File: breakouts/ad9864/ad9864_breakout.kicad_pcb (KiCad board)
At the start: 4 copper layers, 44 x 39 mm, 82 parts, among them P101 CONN_01X02, P102 CONN_01X08, P103 CONN_02X08, U101 CONN_SMA, U102 CONN_SMA, U103 ad9864, U104 TXCO, U105 CONN_SMA, U106 CONN_SMA, U107 max2605

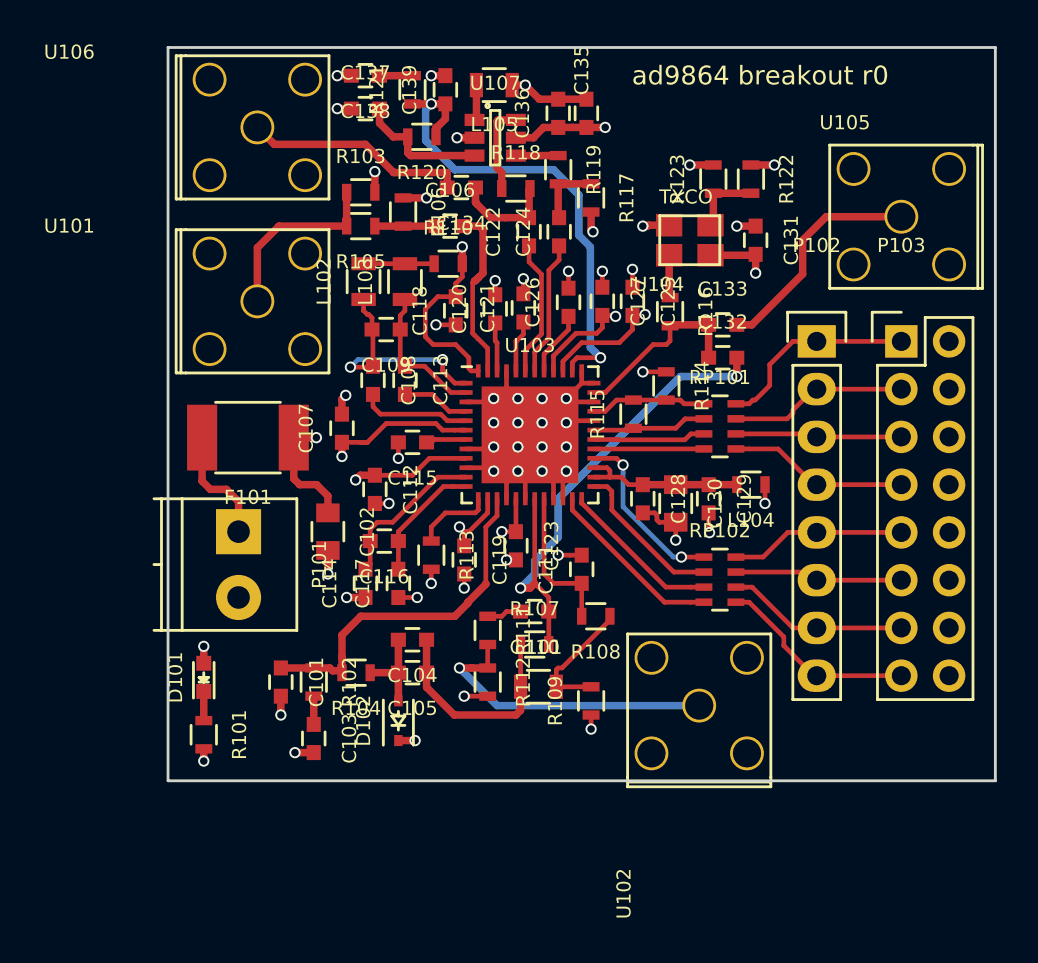
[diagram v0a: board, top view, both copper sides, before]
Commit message: finished ad9864 silkscreen cleanup, ordered r0
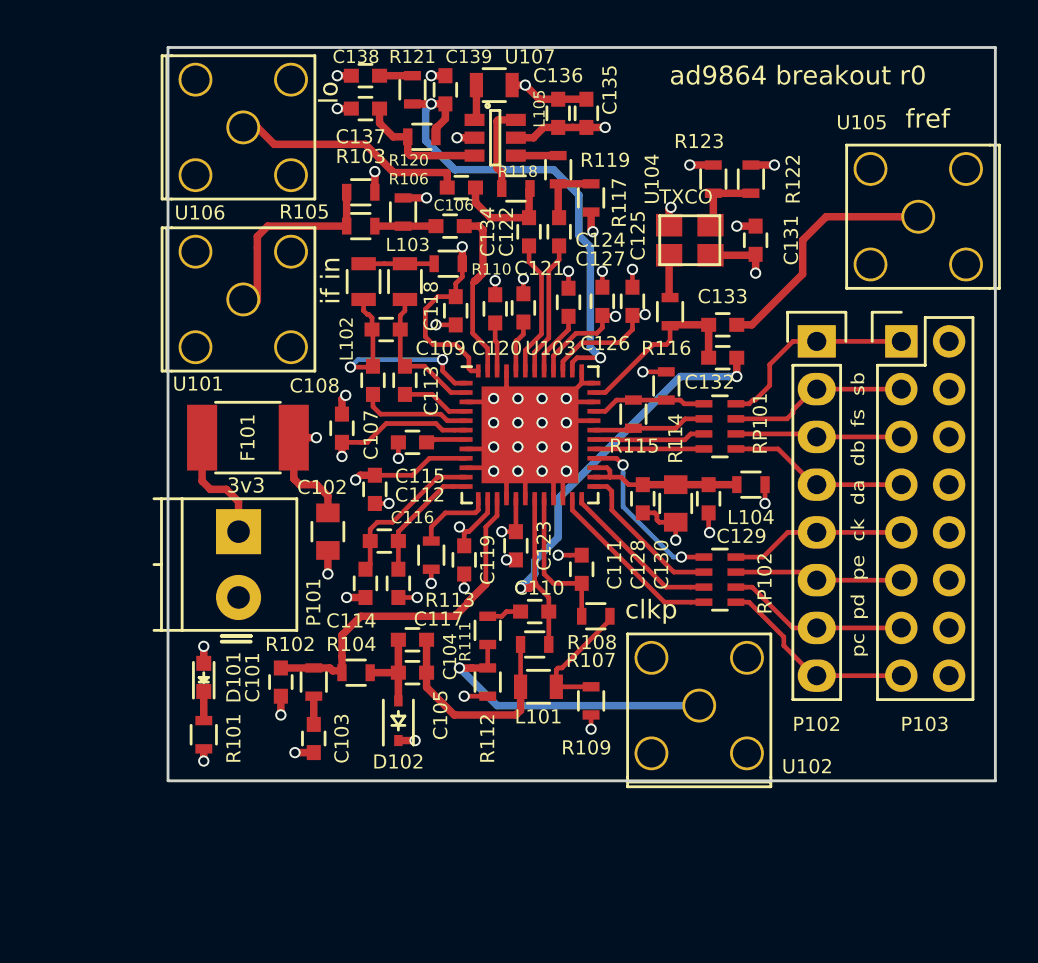
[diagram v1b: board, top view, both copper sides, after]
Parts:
- moved U105 0.90 mm to (151.9, 98.0)
- moved U101 0.76 mm to (116.0, 102.4)
- moved U106 0.75 mm to (116.0, 93.2)
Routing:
- net Net-(C133-Pad2): track 12.2 -> 13.1 mm
- net Net-(C134-Pad2): track 11.9 -> 12.6 mm
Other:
- board text added: "3v3"
- board text added: "clkp"
- board text added: "fref"
- board text added: "if in"
- board text added: "lo"
- board text added: "pc pd pe ck da db fs sb"
